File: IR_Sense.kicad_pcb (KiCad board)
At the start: 2 copper layers, 29.7 x 18.2 mm, 17 parts, among them J1 Conn_01x03, J2 Conn_01x02, Q1 VEMT2020X01, U2 LMV321

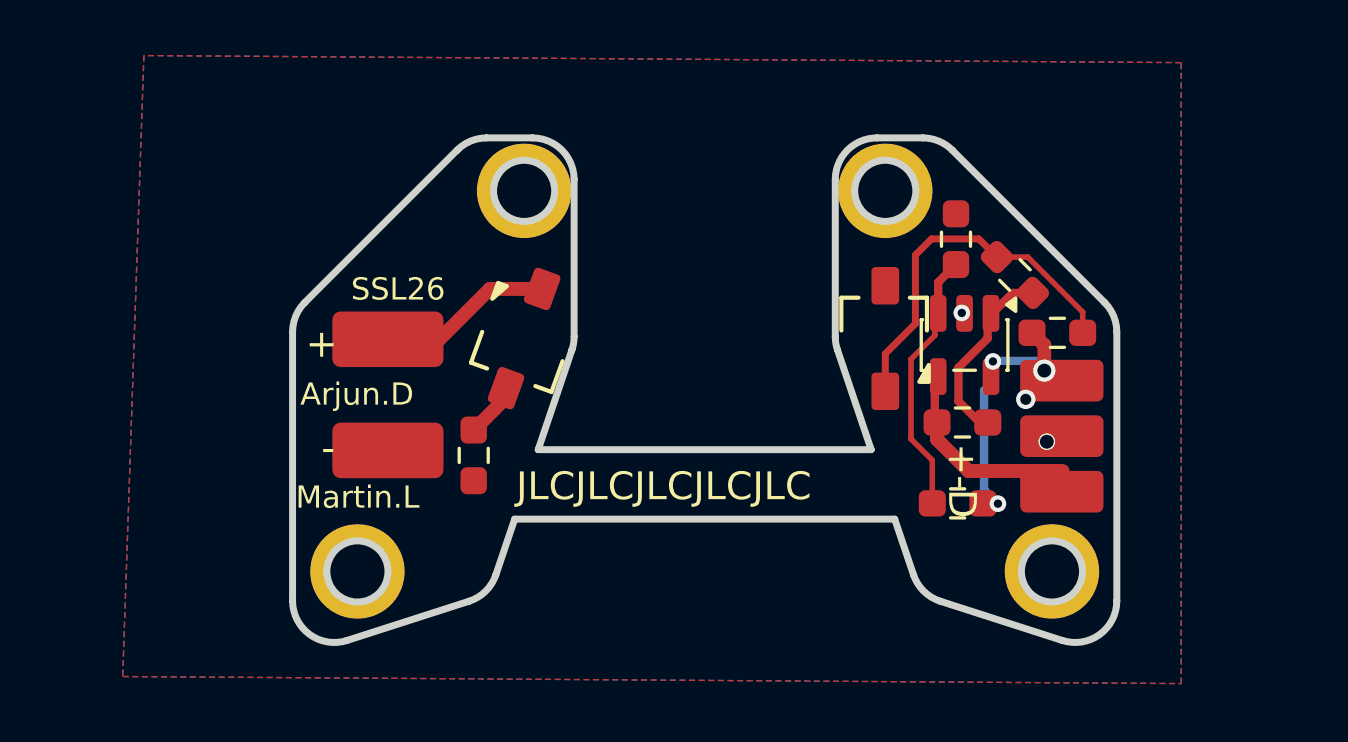
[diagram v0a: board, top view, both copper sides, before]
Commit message: SSL27 refurbish
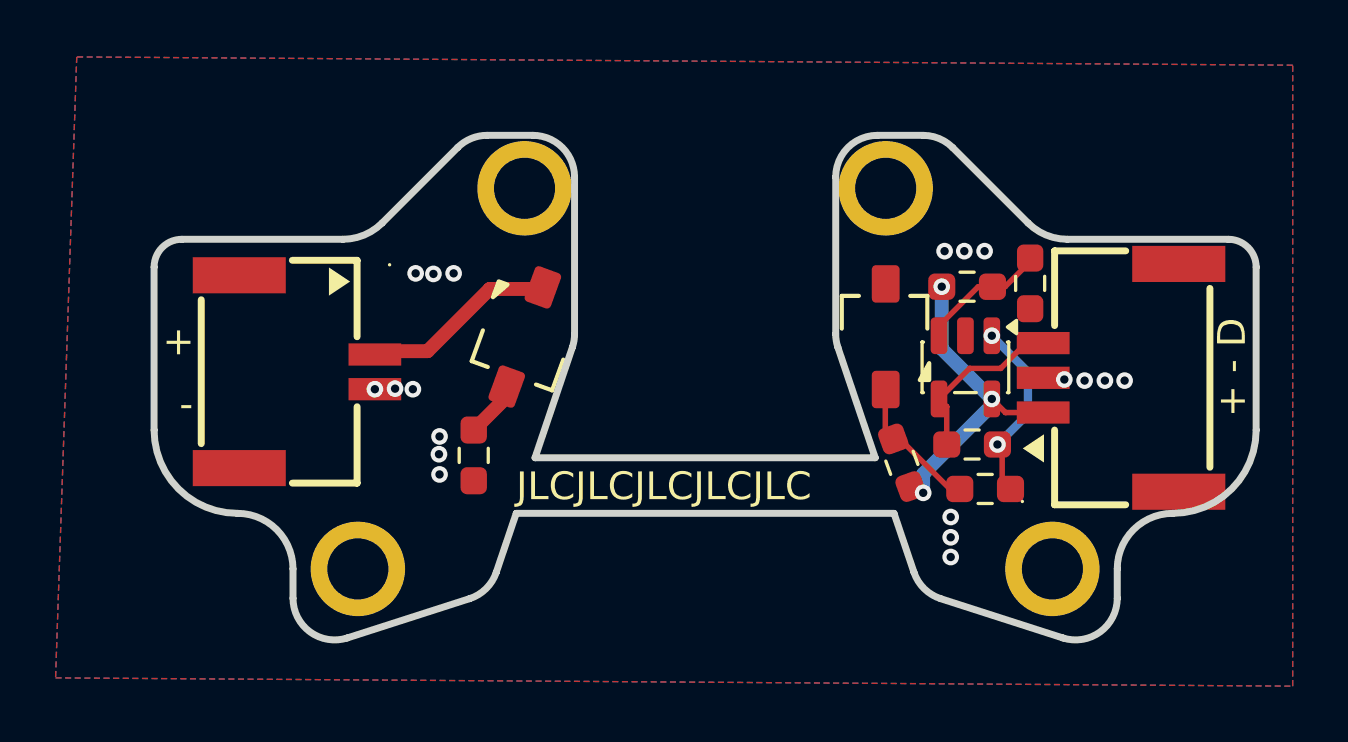
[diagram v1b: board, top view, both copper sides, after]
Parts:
- J1: footprint IR_Sense:J1-SMD_PADS_ONLY -> lcsc:CONN-SMD_3P-P1.25_XUNPU_WAFER-MX1.25-3PCB
- J2: footprint IR_Sense:Tx_Power_Pads -> lcsc:CONN-SMD_2P-P1.25_WAFER-MX1.25-2PCB
- R3: value 150k -> 32k
- R5, R8: value 100k -> 3k
- R6: value 470k -> 66k
- R7: value 100k -> 5.6k
- moved R7 7.81 mm to (103.8, 71.8), turned to 180 degrees
- moved R5 7.77 mm to (104.5, 79.1), turned to 0 degrees
- moved R3 7.29 mm to (101.5, 78.2), turned to 110 degrees
- moved R8 3.11 mm to (106.1, 71.7), turned to 90 degrees
- moved J2 3.03 mm to (80.0, 74.9)
- moved G*** 2.86 mm to (81.4, 74.7)
- moved J1 2.75 mm to (109.0, 75.1)
- moved G*** 2.66 mm to (106.9, 74.9), turned to 180 degrees
- moved R6 0.87 mm to (104.0, 77.5)
- moved U2 0.81 mm to (103.7, 74.7)
- moved H1 0.09 mm to (106.9, 82.0)
- moved H2 0.09 mm to (87.9, 68.3)
- moved H3 0.09 mm to (100.9, 68.3)
- moved H4 0.09 mm to (81.9, 82.0)
- moved Q1 0.07 mm to (100.9, 73.6)
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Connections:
- H1 pad 1: GND -> unconnected-(H1-Pad1)
- H2 pad 1: GND -> unconnected-(H2-Pad1)
- H3 pad 1: GND -> unconnected-(H3-Pad1)
- H4 pad 1: GND -> unconnected-(H4-Pad1)
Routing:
- net Net-(Q1-C): track 13.5 -> 4.98 mm
- net Net-(R7-Pad1): track 9.42 -> 4.58 mm
- net +3.3V: track 10.1 -> 11.2 mm, vias 4 -> 3
- net +5V: track 6.30 -> 7.31 mm
- net IR I/O: track 7.30 -> 6.34 mm
- net Net-(R5-Pad2): track 7.49 -> 6.70 mm, vias 0 -> 2
- net GND: track 0.01 -> 0.00 mm, vias 2 -> 19
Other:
- board size 29.7 x 18.2 mm -> 39.7 x 18.2 mm
- board text added: "+ - D"
- board text added: "IR-RX"
- board text added: "IR-TX"
- board text added: "IRD"
- board text added: "M2"
- board text removed: "+-D"
- board text removed: "Arjun.D"
- board text removed: "IRIO"
- board text removed: "Martin.L"
- board text removed: "SSL26"
